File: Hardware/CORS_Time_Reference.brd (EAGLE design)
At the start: 152.4 x 101.6 mm, 395 parts, among them J10 ANTENNA-SMA-GROUNDEDEDGE_SMA, J11 Vertical Qwiic Connector, J2 ANTENNA-SMA-GROUNDEDEDGE_SMA, J3 MICRO-SD-PUSH-PUSH-EXT-PIN, J4 Vertical Qwiic Connector, J7 ANTENNA-SMA-GROUNDEDEDGE_SMA, J9 MAGJACK-POE, U1 ESP-WROOM-32E, U10 POE_PSU-DP990X, U11 OPA344, U13 OPA344, U2 CH340C, U3 XC6222B331MR-G, U4 U-BLOX_ZED-F9P, U5 ATECC608A, U6 XC6222B331MR-G, U7 W5500, U8 ADC8045, U9 74HC4066_QUAD_BILATERAL_SWITC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, Y1 25MHz

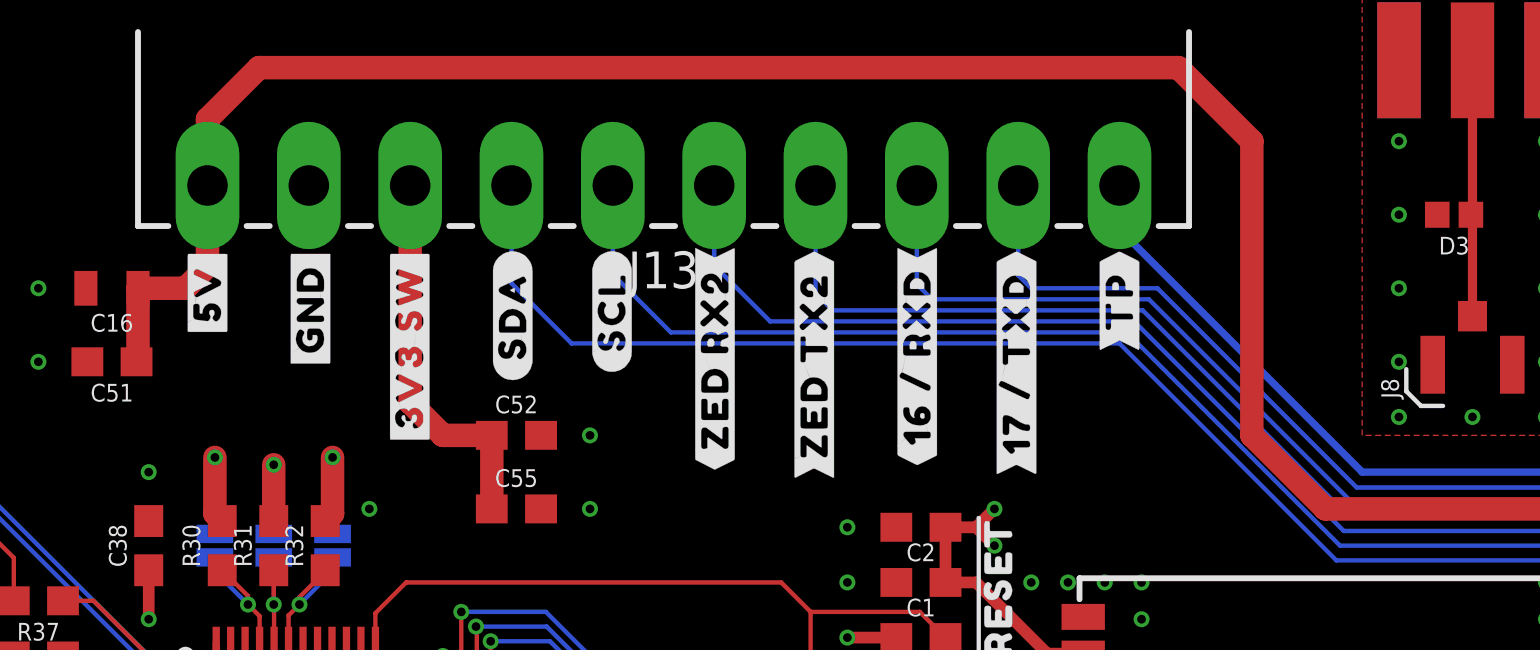
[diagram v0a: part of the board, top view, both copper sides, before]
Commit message: Add CONN-17279
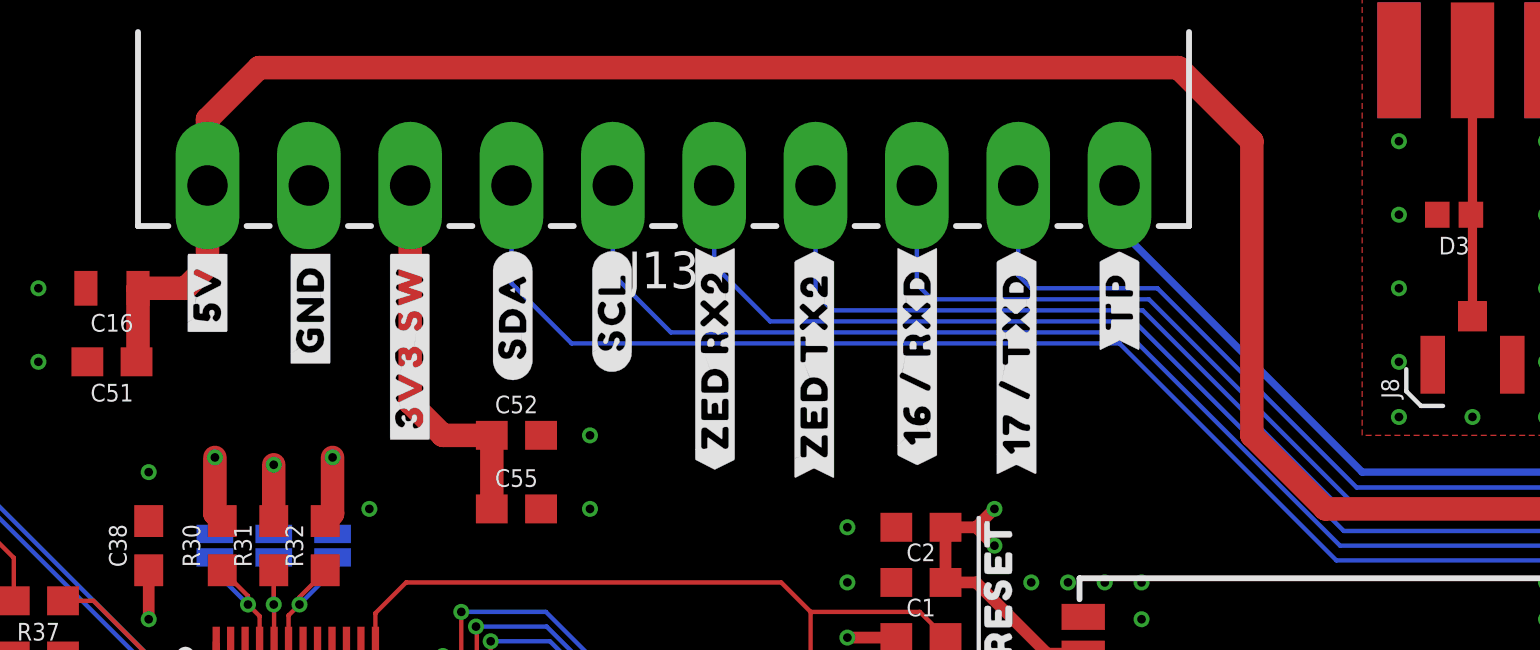
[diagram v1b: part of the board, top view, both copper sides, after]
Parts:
- J13: device Terminal_Connectors:1X10_SCREW_TERMINAL_3.5MM -> SparkFun-Connectors:1X10_SCREW_TERMINAL_3.5MM
